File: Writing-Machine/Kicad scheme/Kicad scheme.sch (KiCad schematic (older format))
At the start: 8 parts

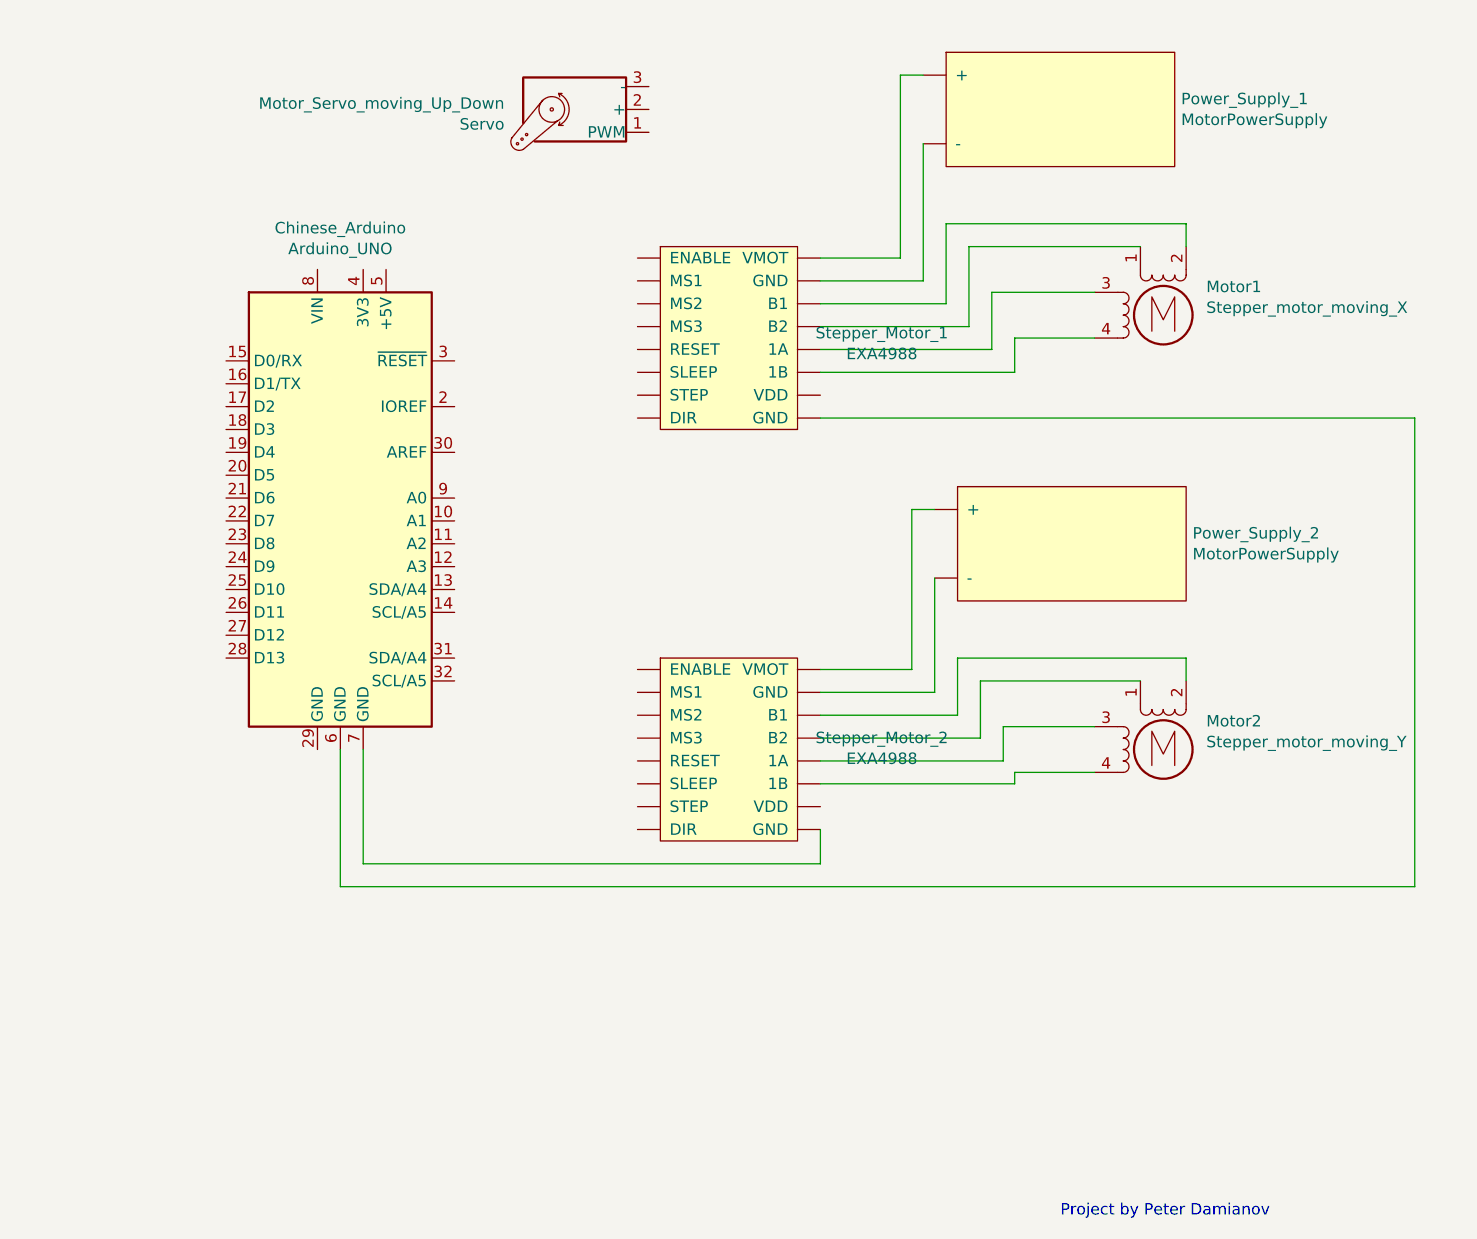
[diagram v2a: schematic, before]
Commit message: Add working scheme
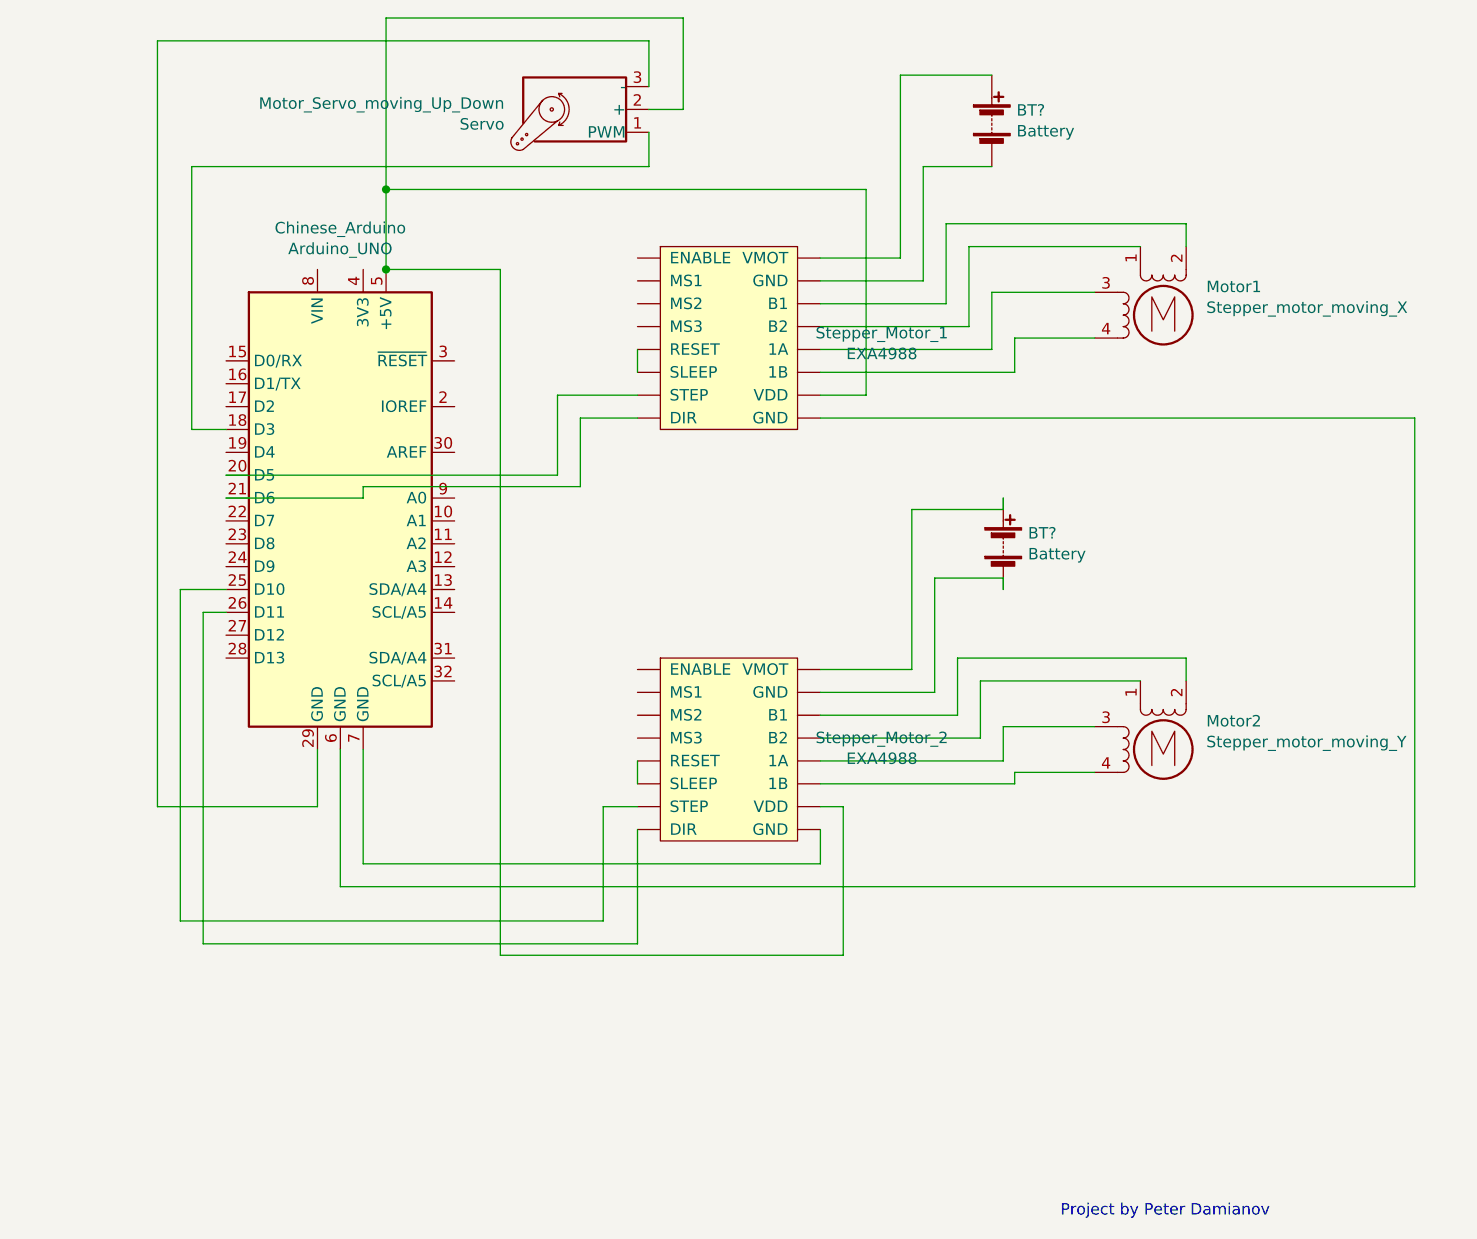
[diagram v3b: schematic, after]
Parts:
- removed Power_Supply_1, Power_Supply_2: MotorPowerSupply, symbol Test:MotorPowerSupply
- added BT? (x2): Battery, symbol Device:Battery
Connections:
- net at Chinese_Arduino.18 (D3): now also Servo.1 (PWM)
- net at Chinese_Arduino.20 (D5): now also Stepper_Motor_1.~ (VMOT)
- net at Chinese_Arduino.21 (D6): now also Stepper_Motor_1.~ (VMOT)
- net at Chinese_Arduino.25 (D10): now also Stepper_Motor_2.~ (VMOT)
- net at Chinese_Arduino.26 (D11): now also Stepper_Motor_2.~ (VMOT)
- net at Chinese_Arduino.29 (GND): now also Servo.3 (-)
- net at Chinese_Arduino.5 (+5V): now also Servo.2 (+), Stepper_Motor_1.~ (VMOT), Stepper_Motor_2.~ (VMOT)
- net at Stepper_Motor_1.~ (VMOT): now also BT?.2 (-)
- net at Stepper_Motor_2.~ (VMOT): now also BT?.2 (-)
- new net: BT?.1 (+), Stepper_Motor_1.~ (VMOT)
- new net: BT?.1 (+), Stepper_Motor_2.~ (VMOT)
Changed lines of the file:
@@
-$EndComp
-$Comp
-L Motor:Stepper_Motor_bipolar Motor2
-U 1 1 5FF2EFA1
-P 7450 4600
-F 0 "Motor2" H 7638 4724 50  0000 L CNN
-F 1 "Stepper_motor_moving_Y" H 7638 4633 50  0000 L CNN
-F 2 "" H 7460 4590 50  0001 C CNN
-F 3 "http://www.infineon.com/dgdl/Application-Note-TLE8110EE_driving_UniPolarStepperMotor_V1.1.pdf?fileId=db3a30431be39b97011be5d0aa0a00b0" H 7460 4590 50  0001 C CNN
-	1    7450 4600
-	1    0    0    -1
 $EndComp
 $Comp
@@
 	6800 2800 6800 2950
 Wire Wire Line
-	6800 2950 5950 2950
-Wire Wire Line
-	7150 4500 6750 4500
-Wire Wire Line
 	6750 4500 6750 4650
 Wire Wire Line
 	6750 4650 5950 4650
 Wire Wire Line
-	7350 4300 6650 4300
-Wire Wire Line
 	6650 4300 6650 4550
 Wire Wire Line
 	6650 4550 5950 4550
-Wire Wire Line
-	7550 4300 7550 4200
-Wire Wire Line
-	7550 4200 6550 4200
 Wire Wire Line
 	6550 4200 6550 4450
@@
 Wire Wire Line
 	6800 4750 5950 4750
-$Comp
-L Test:MotorPowerSupply Power_Supply_1
-U 1 1 6003464B
-P 7000 1800
-F 0 "Power_Supply_1" H 7528 1846 50  0000 L CNN
-F 1 "MotorPowerSupply" H 7528 1755 50  0000 L CNN
-F 2 "" H 7000 1800 50  0001 C CNN
-F 3 "" H 7000 1800 50  0001 C CNN
-	1    7000 1800
-	1    0    0    -1
-$EndComp
-$Comp
-L Test:MotorPowerSupply Power_Supply_2
-U 1 1 60036794
-P 7050 3700
-F 0 "Power_Supply_2" H 7578 3746 50  0000 L CNN
-F 1 "MotorPowerSupply" H 7578 3655 50  0000 L CNN
-F 2 "" H 7050 3700 50  0001 C CNN
-F 3 "" H 7050 3700 50  0001 C CNN
-	1    7050 3700
-	1    0    0    -1
-$EndComp
 Wire Wire Line
 	6450 3850 6450 4350
@@
 	6450 4350 5950 4350
 Wire Wire Line
-	6450 3550 6350 3550
-Wire Wire Line
-	6350 3550 6350 4250
-Wire Wire Line
 	6350 4250 5950 4250
 Wire Wire Line
-	6400 1650 6300 1650
-Wire Wire Line
-	6300 1650 6300 2450
-Wire Wire Line
 	6300 2450 5950 2450
-Wire Wire Line
-	6400 1950 6400 2550
 Wire Wire Line
 	6400 2550 5950 2550
@@
 Text Notes 7000 6650 0    50   ~ 0
 Project by Peter Damianov
+$Comp
+L Device:Battery BT?
+U 1 1 601415E5
+P 6700 1850
+F 0 "BT?" H 6808 1896 50  0000 L CNN
+F 1 "Battery" H 6808 1805 50  0000 L CNN
+F 2 "" V 6700 1910 50  0001 C CNN
+F 3 "~" V 6700 1910 50  0001 C CNN
+	1    6700 1850
+	1    0    0    -1
+$EndComp
+Wire Wire Line
+	6700 2050 6400 2050
+Wire Wire Line
+	6400 2050 6400 2550
+Wire Wire Line
+	6300 2450 6300 1650
+Wire Wire Line
+	6300 1650 6700 1650
+Wire Wire Line
+	6800 2950 5950 2950
+Wire Wire Line
+	7550 4200 6550 4200
+Wire Wire Line
+	7550 4300 7550 4200
+Wire Wire Line
+	7350 4300 6650 4300
+Wire Wire Line
+	7150 4500 6750 4500
+$Comp
+L Motor:Stepper_Motor_bipolar Motor2
+U 1 1 5FF2EFA1
+P 7450 4600
+F 0 "Motor2" H 7638 4724 50  0000 L CNN
+F 1 "Stepper_motor_moving_Y" H 7638 4633 50  0000 L CNN
+F 2 "" H 7460 4590 50  0001 C CNN
+F 3 "http://www.infineon.com/dgdl/Application-Note-TLE8110EE_driving_UniPolarStepperMotor_V1.1.pdf?fileId=db3a30431be39b97011be5d0aa0a00b0" H 7460 4590 50  0001 C CNN
+	1    7450 4600
+	1    0    0    -1
+$EndComp
+$Comp
+L Device:Battery BT?
+U 1 1 60150F60
+P 6750 3700
+F 0 "BT?" H 6858 3746 50  0000 L CNN
+F 1 "Battery" H 6858 3655 50  0000 L CNN
+F 2 "" V 6750 3760 50  0001 C CNN
+F 3 "~" V 6750 3760 50  0001 C CNN
+	1    6750 3700
+	1    0    0    -1
+$EndComp
+Wire Wire Line
+	6450 3850 6750 3850
+Wire Wire Line
+	6750 3850 6750 3900
+Wire Wire Line
+	6750 3550 6750 3500
+Wire Wire Line
+	6350 3550 6750 3550
+Wire Wire Line
+	4050 1400 5350 1400
+Wire Wire Line
+	5350 1400 5350 1800
+Wire Wire Line
+	5350 1800 5200 1800
+Wire Wire Line
+	3350 3200 3200 3200
+Wire Wire Line
+	3200 3200 3200 2050
+Wire Wire Line
+	3200 2050 5200 2050
+Wire Wire Line
+	5200 2050 5200 1900
+Wire Wire Line
+	5200 1700 5200 1500
+Wire Wire Line
+	5200 1500 3050 1500
+Wire Wire Line
+	3050 1500 3050 4850
+Wire Wire Line
+	3750 4850 3750 4600
+Wire Wire Line
+	4800 3400 4800 3050
+Wire Wire Line
+	4800 3050 5150 3050
+Wire Wire Line
+	5150 3150 4900 3150
+Wire Wire Line
+	5150 2950 5150 2850
+Wire Wire Line
+	5150 4750 5150 4650
+Wire Wire Line
+	4050 2500 4050 2150
+Wire Wire Line
+	4550 2500 4550 5500
+Wire Wire Line
+	4550 5500 6050 5500
+Wire Wire Line
+	6050 5500 6050 4850
+Wire Wire Line
+	6050 4850 5950 4850
+Wire Wire Line
+	4050 2150 6150 2150
+Wire Wire Line
+	6150 2150 6150 3050
+Wire Wire Line
+	6150 3050 5950 3050
+Connection ~ 4050 2150
+Wire Wire Line
+	4050 2150 4050 1400
+Wire Wire Line
+	6350 3550 6350 4250
+Wire Wire Line
+	3050 4850 3750 4850
+Wire Wire Line
+	3350 3900 3150 3900
+Wire Wire Line
+	3150 3900 3150 5350
+Wire Wire Line
+	3150 5350 5000 5350
+Wire Wire Line
+	5000 5350 5000 4850
+Wire Wire Line
+	5000 4850 5150 4850
+Wire Wire Line
+	3350 4000 3250 4000
+Wire Wire Line
+	3250 4000 3250 5450
+Wire Wire Line
+	3250 5450 5150 5450
+Wire Wire Line
+	5150 5450 5150 4950
+Connection ~ 4050 2500
+Wire Wire Line
+	3350 3400 4800 3400
+Wire Wire Line
+	4050 2500 4550 2500
+Wire Wire Line
+	3350 3500 3950 3500
+Wire Wire Line
+	3950 3500 3950 3450
+Wire Wire Line
+	4900 3450 4900 3150
+Wire Wire Line
+	3950 3450 4900 3450
 $EndSCHEMATC
